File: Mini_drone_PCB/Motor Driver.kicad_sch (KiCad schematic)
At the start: 16 parts, among them J4 Motor1_Pogo, J5 Motor2_Pogo, J6 Motor3_Pogo, J7 Motor4_Pogo, Q3 AO3400, Q4 AO3400, Q5 AO3400, Q6 AO3400

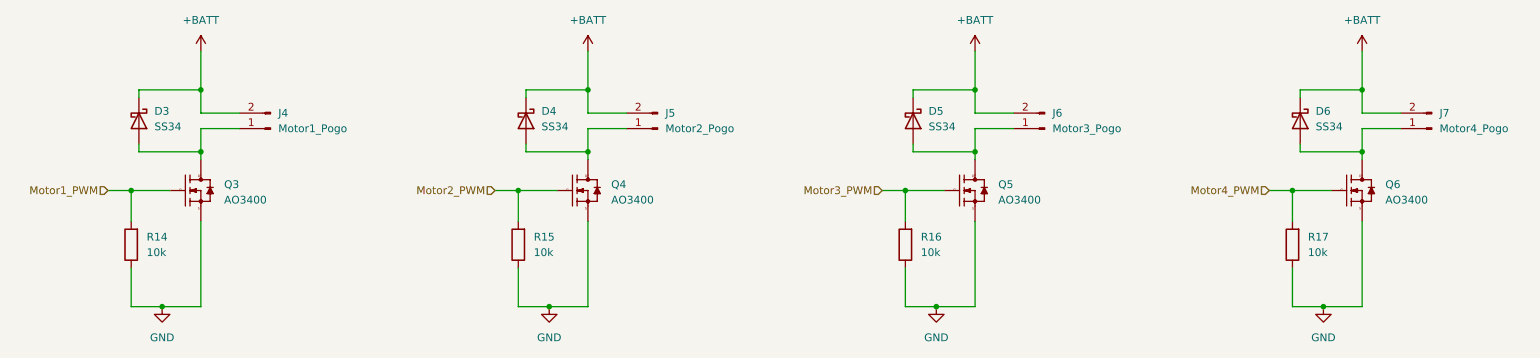
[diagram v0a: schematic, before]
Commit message: Route_Finished
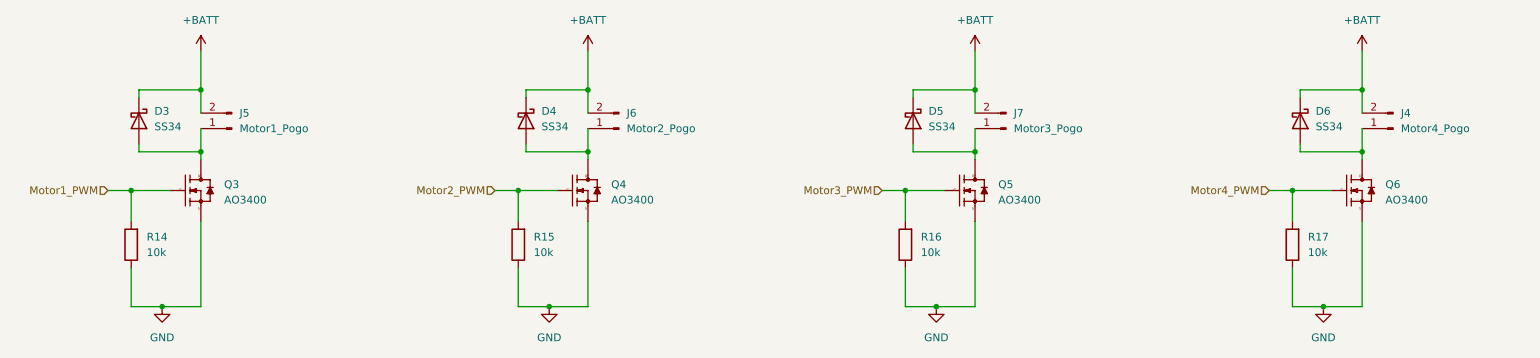
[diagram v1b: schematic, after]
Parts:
- J4: value Motor1_Pogo -> Motor4_Pogo; footprint (none) -> mini_drone:POGO 2Pin Pitch 4
- J5: value Motor2_Pogo -> Motor1_Pogo; footprint (none) -> mini_drone:POGO 2Pin Pitch 4
- J6: value Motor3_Pogo -> Motor2_Pogo; footprint (none) -> mini_drone:POGO 2Pin Pitch 4
- J7: value Motor4_Pogo -> Motor3_Pogo; footprint (none) -> mini_drone:POGO 2Pin Pitch 4
- R14, R15, R16, R17: LCSC Part # C25531 -> C25531
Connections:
- net at D5.2 (A), Q5.3 (D): now also J7.1 (Pin_1); no longer J6.1 (Pin_1)
- net at D4.2 (A), Q4.3 (D): now also J6.1 (Pin_1); no longer J5.1 (Pin_1)
- net at D3.2 (A), Q3.3 (D): now also J5.1 (Pin_1); no longer J4.1 (Pin_1)
- net at D6.2 (A), Q6.3 (D): now also J4.1 (Pin_1); no longer J7.1 (Pin_1)
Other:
- moved on the sheet: J4, J5, J6, J7
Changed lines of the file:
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@@
-	(wire
-		(pts
-			(xy 185.42 90.17) (xy 191.77 90.17)
-		)
-		(stroke
-			(width 0)
-			(type default)
-		)
-	)
 	(wire
 		(pts
@@
 	(wire
 		(pts
-			(xy 255.27 87.63) (xy 248.92 87.63)
-		)
-		(stroke
-			(width 0)
-			(type default)
-		)
-	)
-	(wire
-		(pts
 			(xy 237.49 100.33) (xy 243.84 100.33)
 		)
@@
 	(wire
 		(pts
-			(xy 191.77 87.63) (xy 185.42 87.63)
-		)
-		(stroke
-			(width 0)
-			(type default)
-		)
-	)
-	(wire
-		(pts
-			(xy 58.42 90.17) (xy 64.77 90.17)
-		)
-		(stroke
-			(width 0)
-			(type default)
-		)
-	)
-	(wire
-		(pts
-			(xy 64.77 87.63) (xy 58.42 87.63)
-		)
-		(stroke
-			(width 0)
-			(type default)
-		)
-	)
-	(wire
-		(pts
 			(xy 58.42 77.47) (xy 58.42 83.82)
 		)
@@
 	(wire
 		(pts
-			(xy 248.92 90.17) (xy 255.27 90.17)
-		)
-		(stroke
-			(width 0)
-			(type default)
-		)
-	)
-	(wire
-		(pts
 			(xy 48.26 93.98) (xy 58.42 93.98)
 		)
@@
 		(pts
 			(xy 179.07 119.38) (xy 185.42 119.38)
-		)
-		(stroke
-			(width 0)
-			(type default)
-		)
-	)
-	(wire
-		(pts
-			(xy 128.27 87.63) (xy 121.92 87.63)
-		)
-		(stroke
-			(width 0)
-			(type default)
-		)
-	)
-	(wire
-		(pts
-			(xy 121.92 90.17) (xy 128.27 90.17)
 		)
 		(stroke
@@
 			)
 		)
-		(property "LCSC Part #" " C25531"
+		(property "LCSC Part #" "C25531"
 			(at 237.49 109.22 90)
 			(effects
@@
 	(symbol
 		(lib_id "Connector:Conn_01x02_Pin")
-		(at 69.85 90.17 180)
+		(at 254 90.17 180)
 		(unit 1)
 		(exclude_from_sim no)
@@
 		(fields_autoplaced yes)
 		(property "Reference" "J4"
-			(at 71.12 87.6299 0)
+			(at 255.27 87.6299 0)
 			(effects
 				(font
@@
 			)
 		)
-		(property "Value" "Motor1_Pogo"
-			(at 71.12 90.1699 0)
+		(property "Value" "Motor4_Pogo"
+			(at 255.27 90.1699 0)
 			(effects
 				(font
@@
 			)
 		)
-		(property "Footprint" ""
-			(at 69.85 90.17 0)
+		(property "Footprint" "mini_drone:POGO 2Pin Pitch 4"
+			(at 254 90.17 0)
 			(effects
 				(font
@@
 		)
 		(property "Datasheet" "~"
-			(at 69.85 90.17 0)
+			(at 254 90.17 0)
 			(effects
 				(font
@@
 		)
 		(property "Description" "Generic connector, single row, 01x02, script generated"
-			(at 69.85 90.17 0)
+			(at 254 90.17 0)
 			(effects
 				(font
@@
 	(symbol
 		(lib_id "Connector:Conn_01x02_Pin")
-		(at 133.35 90.17 180)
+		(at 63.5 90.17 180)
 		(unit 1)
 		(exclude_from_sim no)
@@
 		(fields_autoplaced yes)
 		(property "Reference" "J5"
-			(at 134.62 87.6299 0)
+			(at 64.77 87.6299 0)
 			(effects
 				(font
@@
 			)
 		)
-		(property "Value" "Motor2_Pogo"
-			(at 134.62 90.1699 0)
+		(property "Value" "Motor1_Pogo"
+			(at 64.77 90.1699 0)
 			(effects
 				(font
@@
 			)
 		)
-		(property "Footprint" ""
-			(at 133.35 90.17 0)
+		(property "Footprint" "mini_drone:POGO 2Pin Pitch 4"
+			(at 63.5 90.17 0)
 			(effects
 				(font
@@
 		)
 		(property "Datasheet" "~"
-			(at 133.35 90.17 0)
+			(at 63.5 90.17 0)
 			(effects
 				(font
@@
 		)
 		(property "Description" "Generic connector, single row, 01x02, script generated"
-			(at 133.35 90.17 0)
+			(at 63.5 90.17 0)
 			(effects
 				(font
@@
 	(symbol
 		(lib_id "Connector:Conn_01x02_Pin")
-		(at 196.85 90.17 180)
+		(at 127 90.17 180)
 		(unit 1)
 		(exclude_from_sim no)
@@
 		(fields_autoplaced yes)
 		(property "Reference" "J6"
-			(at 198.12 87.6299 0)
+			(at 128.27 87.6299 0)
 			(effects
 				(font
@@
 			)
 		)
-		(property "Value" "Motor3_Pogo"
-			(at 198.12 90.1699 0)
+		(property "Value" "Motor2_Pogo"
+			(at 128.27 90.1699 0)
 			(effects
 				(font
@@
 			)
 		)
-		(property "Footprint" ""
-			(at 196.85 90.17 0)
+		(property "Footprint" "mini_drone:POGO 2Pin Pitch 4"
+			(at 127 90.17 0)
 			(effects
 				(font
@@
 		)
 		(property "Datasheet" "~"
-			(at 196.85 90.17 0)
+			(at 127 90.17 0)
 			(effects
 				(font
@@
 		)
 		(property "Description" "Generic connector, single row, 01x02, script generated"
-			(at 196.85 90.17 0)
+			(at 127 90.17 0)
 			(effects
 				(font
@@
 			)
 		)
-		(property "LCSC Part #" " C25531"
+		(property "LCSC Part #" "C25531"
 			(at 173.99 109.22 90)
 			(effects
@@
 			)
 		)
-		(property "LCSC Part #" " C25531"
+		(property "LCSC Part #" "C25531"
 			(at 46.99 109.22 90)
 			(effects
@@
 	(symbol
 		(lib_id "Connector:Conn_01x02_Pin")
-		(at 260.35 90.17 180)
+		(at 190.5 90.17 180)
 		(unit 1)
 		(exclude_from_sim no)
@@
 		(fields_autoplaced yes)
 		(property "Reference" "J7"
-			(at 261.62 87.6299 0)
+			(at 191.77 87.6299 0)
 			(effects
 				(font
@@
 			)
 		)
-		(property "Value" "Motor4_Pogo"
-			(at 261.62 90.1699 0)
+		(property "Value" "Motor3_Pogo"
+			(at 191.77 90.1699 0)
 			(effects
 				(font
@@
 			)
 		)
-		(property "Footprint" ""
-			(at 260.35 90.17 0)
+		(property "Footprint" "mini_drone:POGO 2Pin Pitch 4"
+			(at 190.5 90.17 0)
 			(effects
 				(font
@@
 		)
 		(property "Datasheet" "~"
-			(at 260.35 90.17 0)
+			(at 190.5 90.17 0)
 			(effects
 				(font
@@
 		)
 		(property "Description" "Generic connector, single row, 01x02, script generated"
-			(at 260.35 90.17 0)
+			(at 190.5 90.17 0)
 			(effects
 				(font
@@
 			)
 		)
-		(property "LCSC Part #" " C25531"
+		(property "LCSC Part #" "C25531"
 			(at 110.49 109.22 90)
 			(effects
